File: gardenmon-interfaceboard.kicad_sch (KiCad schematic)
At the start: 29 parts, among them J1 Conn_02x20_Odd_Even, J2 Conn_01x04, J3 Conn_01x10, J4 Conn_01x04, J5 Conn_01x04, J6 Conn_01x03

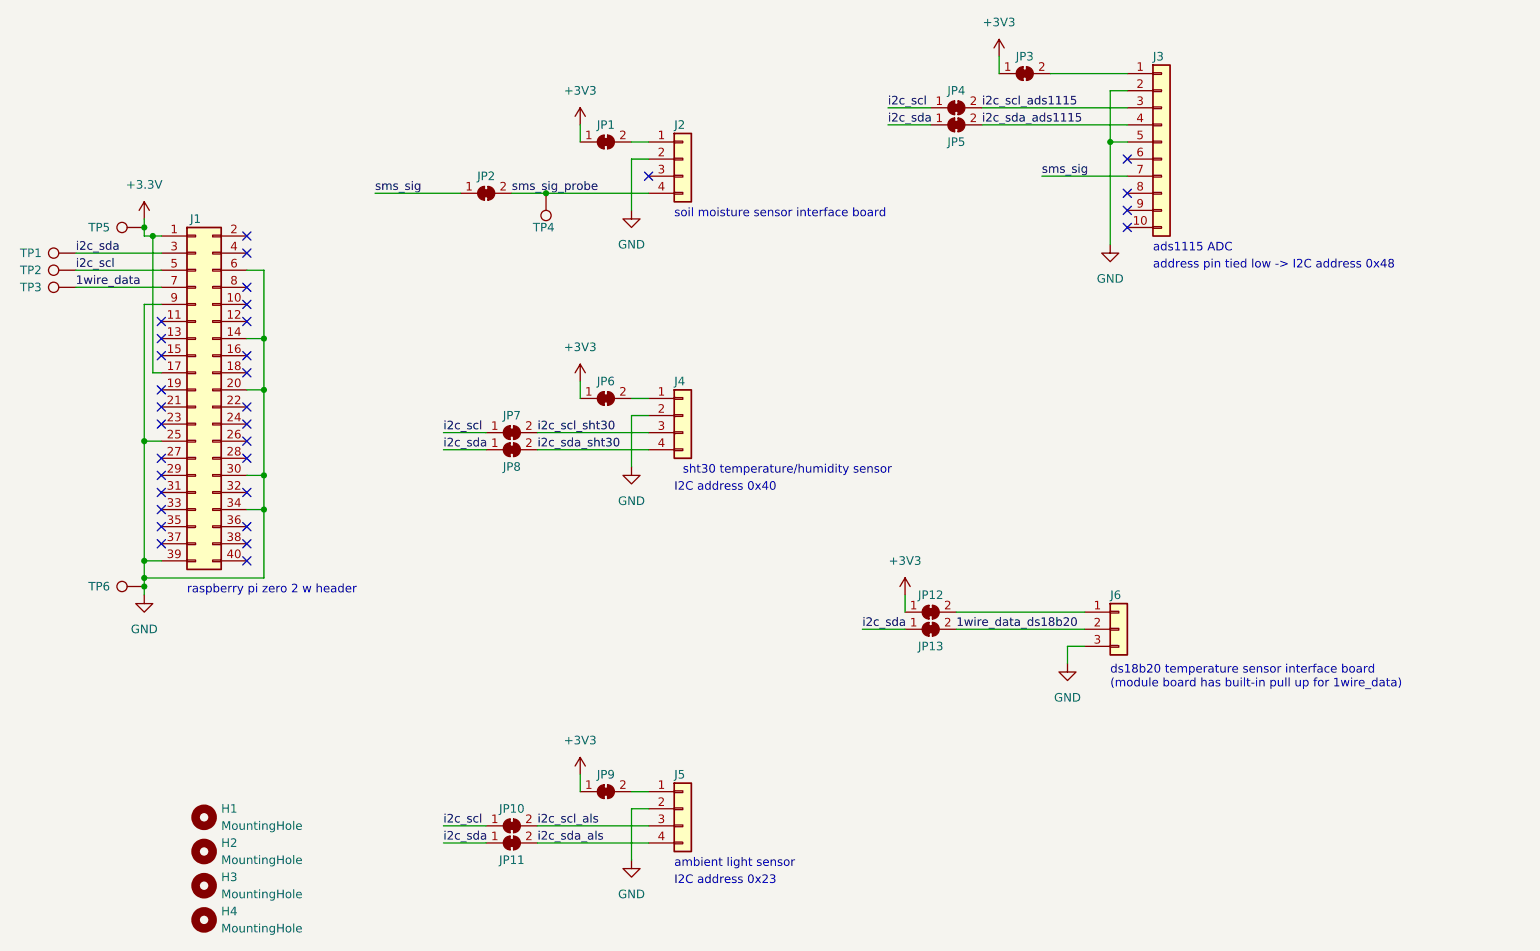
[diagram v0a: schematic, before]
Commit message: temp:
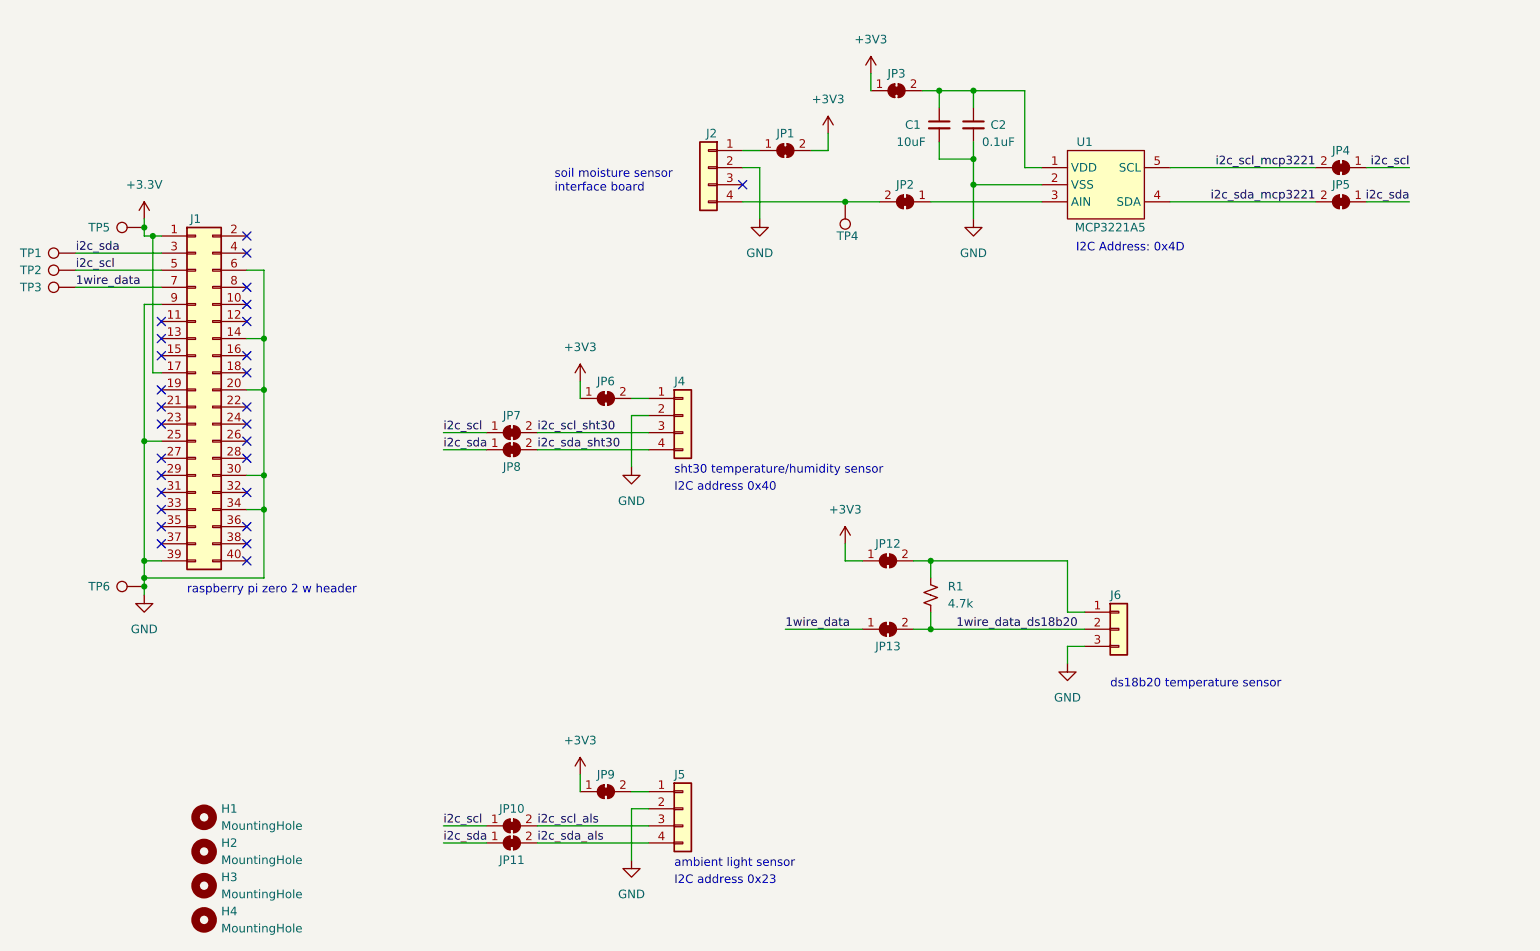
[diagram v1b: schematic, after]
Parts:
- removed J3: Conn_01x10, Connector_PinHeader_2.54mm:PinHeader_1x10_P2.54mm_Vertical, symbol Connector_Generic:Conn_01x10
- added C1: 10uF, Capacitor_SMD:C_0603_1608Metric_Pad1.08x0.95mm_HandSolder, symbol Device:C_Small
- added C2: 0.1uF, Capacitor_SMD:C_0603_1608Metric_Pad1.08x0.95mm_HandSolder, symbol Device:C_Small
- added R1: 4.7k, Resistor_SMD:R_0603_1608Metric_Pad0.98x0.95mm_HandSolder, symbol Device:R_Small_US
- added U1: MCP3221A5, Package_TO_SOT_SMD:SOT-23-5_HandSoldering, symbol gardenmon-interfaceboard:MCP3221A5
- J2, J4, J5: footprint Connector_PinHeader_2.54mm:PinHeader_1x04_P2.54mm_Vertical -> Connector_PinSocket_2.54mm:PinSocket_1x04_P2.54mm_Vertical
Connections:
- net +3V3: now also JP1.2 (B); no longer JP1.1 (A)
- net 1wire_data: now also JP13.1 (A)
- net 1wire_data_ds18b20: now also R1.2
- net GND: now also C1.2, C2.2, U1.2 (VSS)
- net i2c_sda: no longer JP13.1 (A)
- net at J2.1 (Pin_1): now also JP1.1 (A); no longer JP1.2 (B)
- net at JP3.2 (B): now also C1.1, C2.1, U1.1 (VDD)
- net at J6.1 (Pin_1), JP12.2 (B): now also R1.1
- net i2c_scl_ads1115 renamed i2c_scl_mcp3221
- net i2c_scl_mcp3221: now also U1.5 (SCL)
- net i2c_sda_ads1115 renamed i2c_sda_mcp3221
- net i2c_sda_mcp3221: now also U1.4 (SDA)
- net sms_sig: no longer names the net of JP2.1 (A)
- net sms_sig: now also U1.3 (AIN)
- net sms_sig_probe: no longer names the net of J2.4 (Pin_4), JP2.2 (B), TP4.1
- no-connect marks 32 -> 28
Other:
- note added: "I2C Address: 0x4D"
- note added: "ds18b20 temperature sensor"
- note removed: "address pin tied low -> I2C address 0x48"
- note removed: "ads1115 ADC"
- note removed: "ds18b20 temperature sensor interface board (module board has built-in pull up for 1wire_data)"
- moved on the sheet: J2, JP1, JP12, JP13, JP2, JP3, JP4, JP5, TP4
